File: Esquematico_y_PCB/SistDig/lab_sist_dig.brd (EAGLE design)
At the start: 93.8 x 85.2 mm, 25 parts

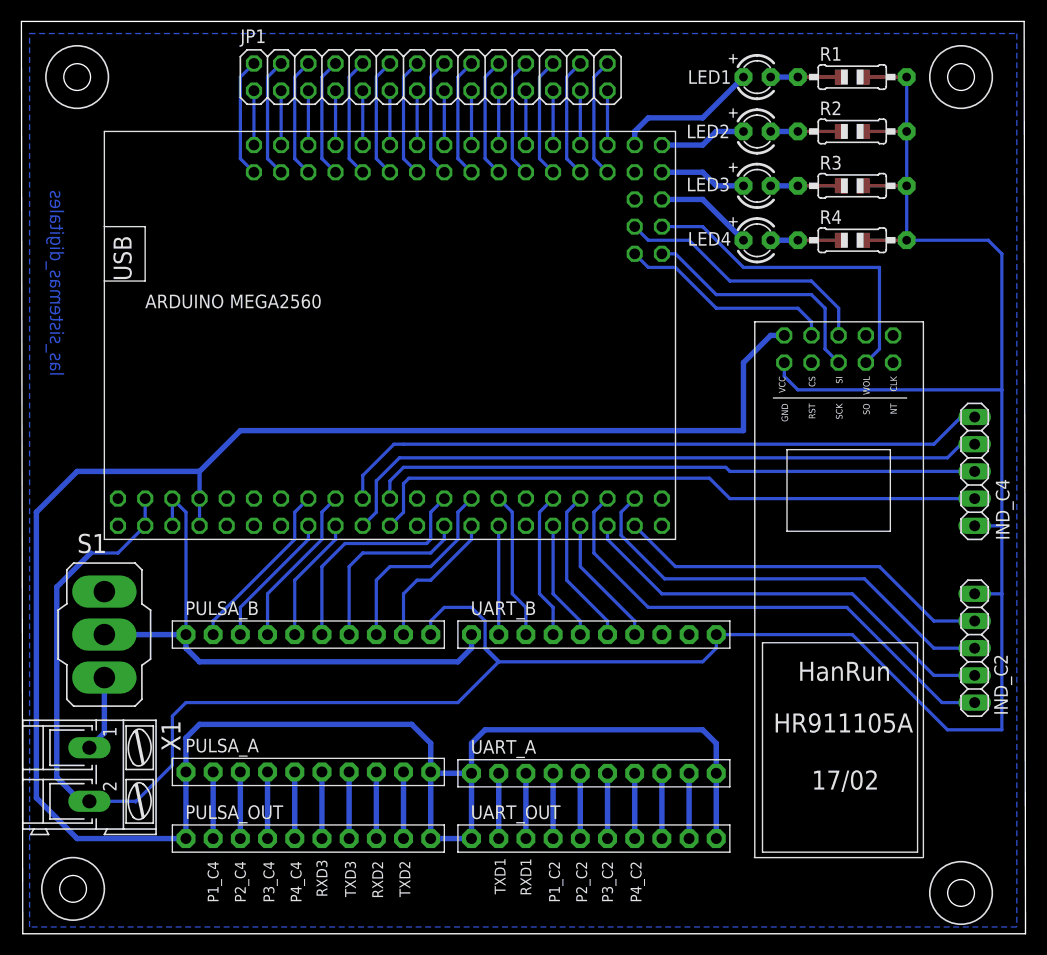
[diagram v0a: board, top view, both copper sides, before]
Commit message: PCB y esquematico
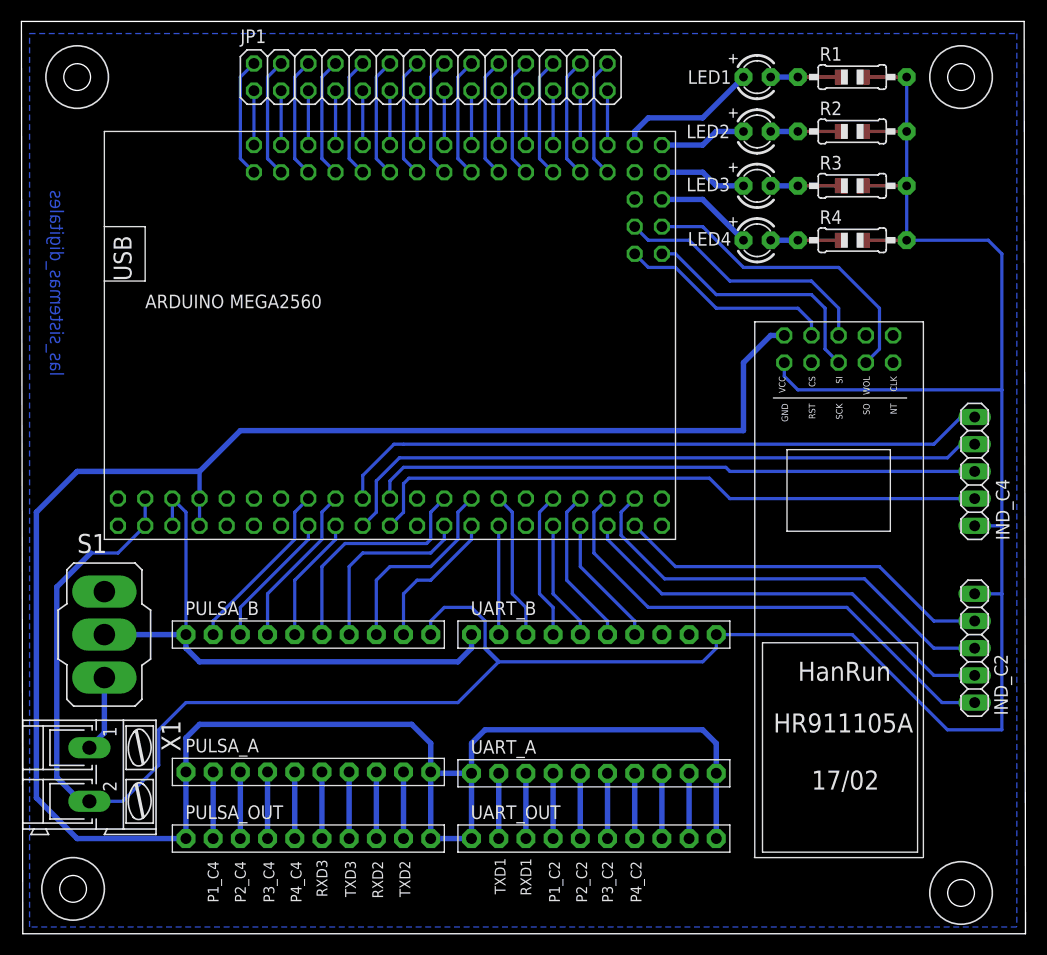
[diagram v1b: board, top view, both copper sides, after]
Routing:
- net SO: track 31.3 -> 29.1 mm
- net GND: track 242.3 -> 241.1 mm
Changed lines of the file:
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@@
 <contactref element="U$2" pad="SO"/>
 <wire x1="76.2" y1="54.61" x2="77.47" y2="55.88" width="0.3048" layer="16"/>
-<wire x1="77.47" y1="63.5" x2="64.77" y2="63.5" width="0.3048" layer="16"/>
 <wire x1="64.77" y1="63.5" x2="60.96" y2="67.31" width="0.3048" layer="16"/>
 <wire x1="60.96" y1="67.31" x2="57.15" y2="67.31" width="0.3048" layer="16"/>
-<wire x1="77.47" y1="55.88" x2="77.47" y2="63.5" width="0.3048" layer="16"/>
+<wire x1="77.47" y1="59.69" x2="77.47" y2="55.88" width="0.3048" layer="16"/>
+<wire x1="64.77" y1="63.5" x2="73.66" y2="63.5" width="0.3048" layer="16"/>
+<wire x1="73.66" y1="63.5" x2="77.47" y2="59.69" width="0.3048" layer="16"/>
 </signal>
 <signal name="SI">
@@
 <wire x1="3.6322" y1="13.589" x2="3.683" y2="13.6398" width="0.3048" layer="16"/>
 <wire x1="0.635" y1="33.655" x2="0.635" y2="15.875" width="0.508" layer="16"/>
-<wire x1="3.683" y1="13.6398" x2="7.9502" y2="13.6398" width="0.3048" layer="16"/>
-<wire x1="7.9502" y1="13.6398" x2="8.001" y2="13.589" width="0.3048" layer="16"/>
-<wire x1="11.43" y1="17.018" x2="11.43" y2="21.59" width="0.3048" layer="16"/>
-<wire x1="11.43" y1="21.59" x2="12.7" y2="22.86" width="0.3048" layer="16"/>
+<wire x1="3.683" y1="13.6398" x2="6.7818" y2="13.6398" width="0.3048" layer="16"/>
+<wire x1="10.16" y1="17.018" x2="10.16" y2="20.32" width="0.3048" layer="16"/>
+<wire x1="10.16" y1="20.32" x2="12.7" y2="22.86" width="0.3048" layer="16"/>
 <wire x1="38.1" y1="22.86" x2="41.91" y2="26.67" width="0.3048" layer="16"/>
-<wire x1="8.001" y1="13.589" x2="11.43" y2="17.018" width="0.3048" layer="16"/>
+<wire x1="6.7818" y1="13.6398" x2="10.16" y2="17.018" width="0.3048" layer="16"/>
 <wire x1="12.7" y1="22.86" x2="38.1" y2="22.86" width="0.3048" layer="16"/>
 <wire x1="80.01" y1="66.04" x2="80.01" y2="71.12" width="0.3048" layer="16"/>
@@
 <wire x1="80.01" y1="81.28" x2="80.01" y2="76.2" width="0.3048" layer="16"/>
 <wire x1="3.683" y1="13.6398" x2="2.8702" y2="13.6398" width="0.508" layer="16"/>
-<wire x1="2.8702" y1="13.6398" x2="2.54" y2="13.97" width="0.508" layer="16"/>
 <wire x1="0.635" y1="15.875" x2="2.8702" y2="13.6398" width="0.508" layer="16"/>
 <polygon width="0.3048" layer="16" isolate="1.27">
